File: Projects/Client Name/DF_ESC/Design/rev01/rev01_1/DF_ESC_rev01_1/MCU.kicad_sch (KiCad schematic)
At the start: 11 parts, among them U1 STM32F405RGTx

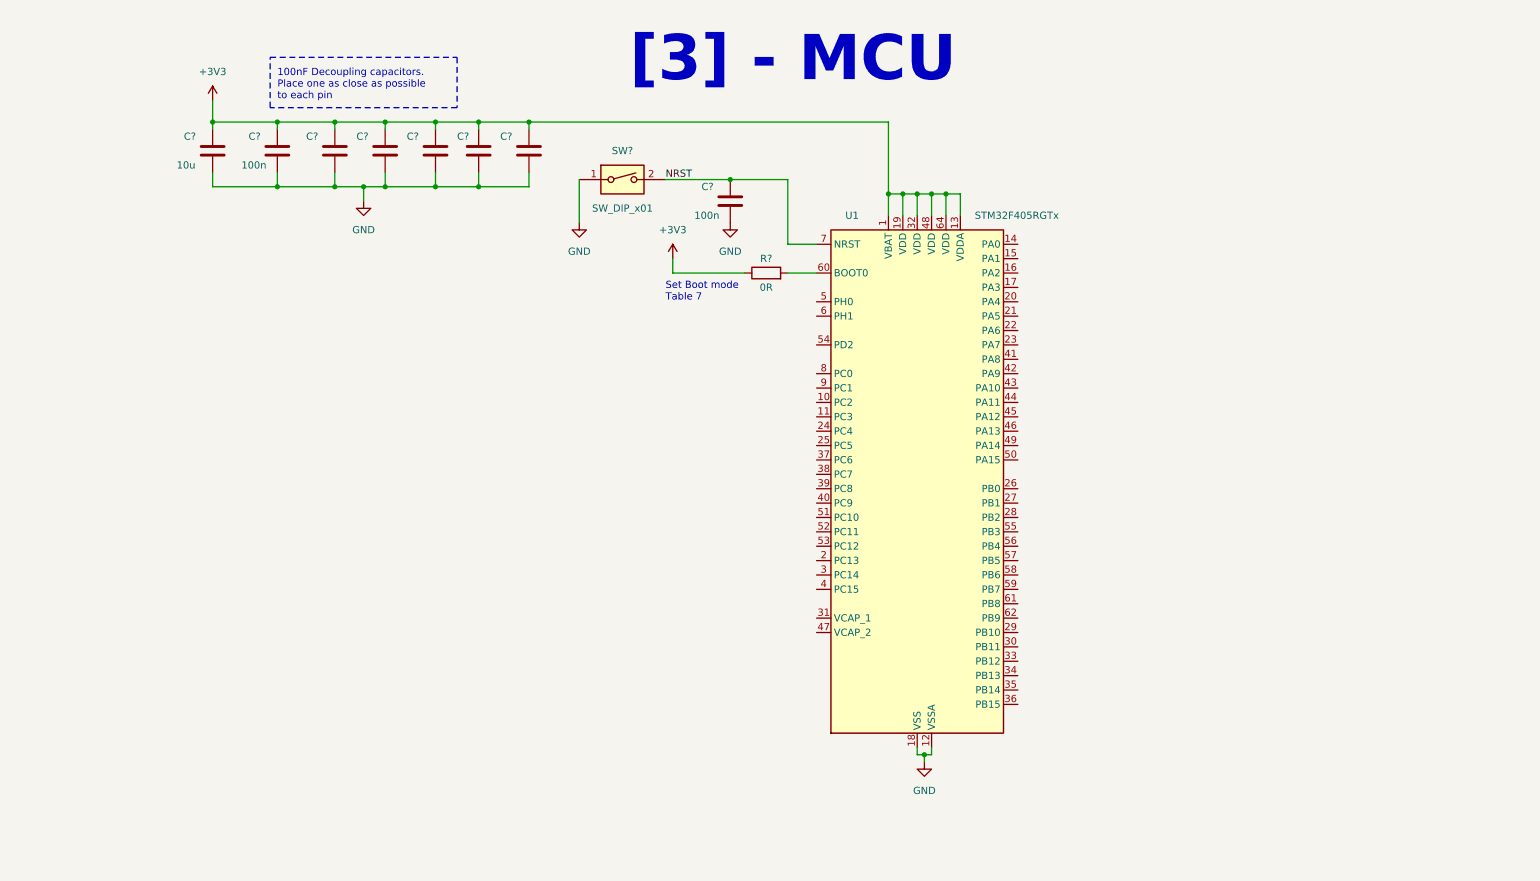
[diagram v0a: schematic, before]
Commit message: Update 19-01-2024_3
MCU schematic complete
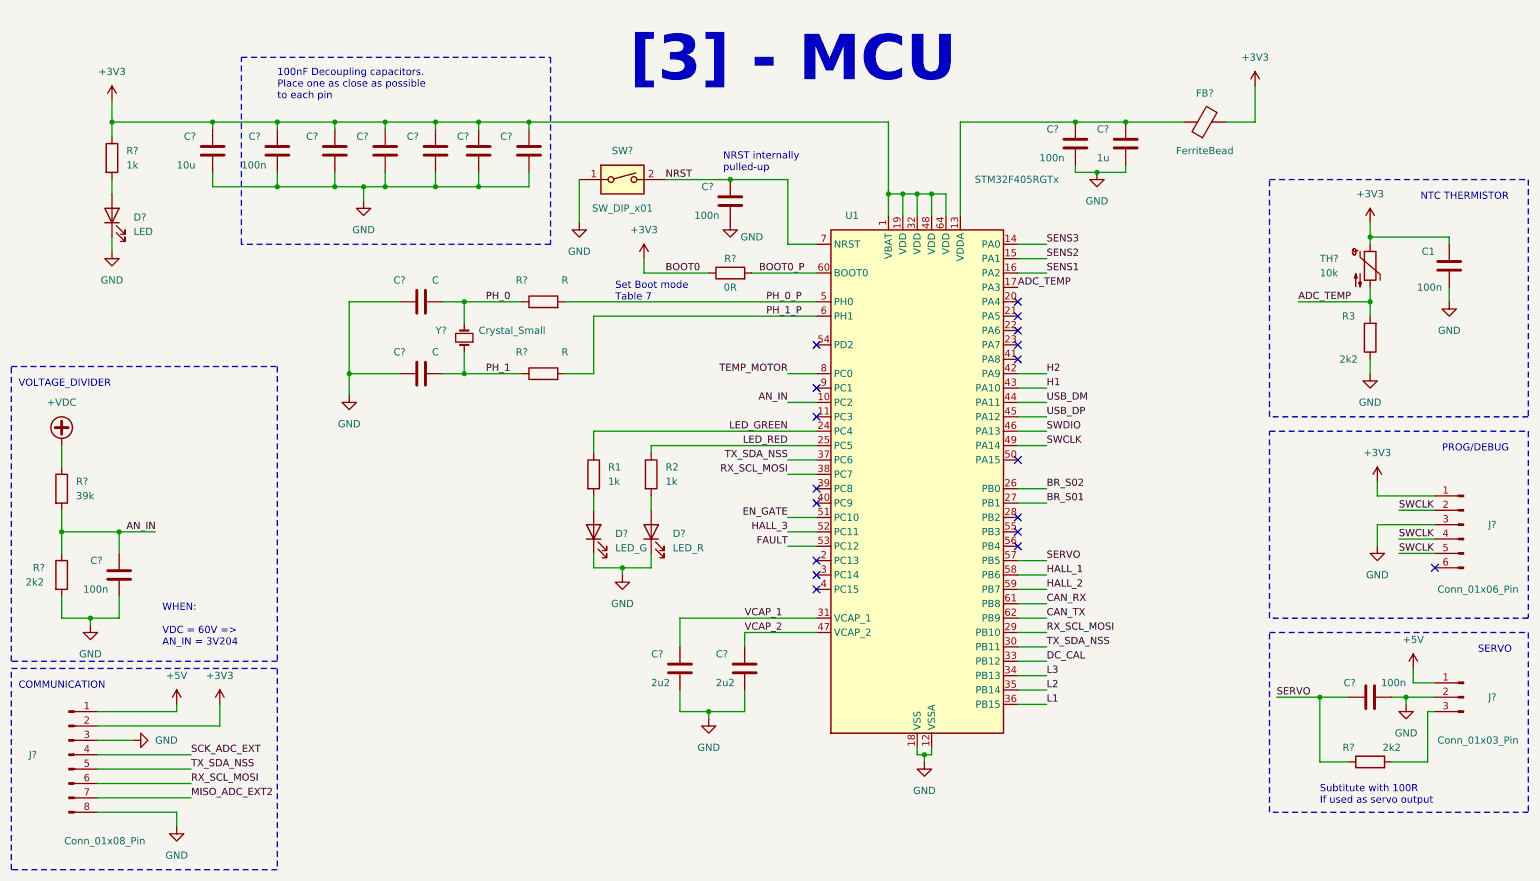
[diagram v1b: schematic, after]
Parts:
- added C1, C? (x3): 100n, symbol Device:C
- added C? (x2): 2u2, symbol Device:C
- added C?: 1u, symbol Device:C
- added C? (x2): C, symbol Device:C
- added D?: LED_G, symbol Device:LED
- added D?: LED_R, symbol Device:LED
- added D?: LED, symbol Device:LED
- added FB?: FerriteBead, symbol Device:FerriteBead
- added J?: Conn_01x03_Pin, symbol Connector:Conn_01x03_Pin
- added J?: Conn_01x08_Pin, symbol Connector:Conn_01x08_Pin
- added J?: Conn_01x06_Pin, symbol Connector:Conn_01x06_Pin
- added R1, R2, R?: 1k, symbol Device:R
- added R3, R? (x2): 2k2, symbol Device:R
- added R?: 39k, symbol Device:R
- added R? (x2): R, symbol Device:R
- added TH?: 10k, symbol Device:Thermistor_NTC
- added Y?: Crystal_Small, symbol Device:Crystal_Small
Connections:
- net +3V3: now also C1.2, FB?.2, J?.1 (Pin_1), J?.2 (Pin_2), R?.1, TH?.1; no longer U1.13 (VDDA)
- net GND: now also C1.1, C?.1, C?.1, C?.2, C?.2, C?.2, C?.2, C?.2, C?.2, D?.1 (K), D?.1 (K), D?.1 (K), J?.2 (Pin_2), J?.3 (Pin_3), J?.3 (Pin_3), J?.8 (Pin_8), R3.1, R?.2
- net BOOT0_P: now reaches R?.2, U1.60 (BOOT0)
- net AN_IN: now reaches U1.10 (PC2)
- net AN_IN: now also C?.1, R?.1, R?.2
- net SENS3: now reaches U1.14 (PA0)
- net SENS2: now reaches U1.15 (PA1)
- net SENS1: now reaches U1.16 (PA2)
- net ADC_TEMP: now reaches U1.17 (PA3)
- net ADC_TEMP: now also R3.2, TH?.2
- net LED_GREEN: now reaches U1.24 (PC4)
- net LED_GREEN: now also R1.1
- net LED_RED: now reaches U1.25 (PC5)
- net LED_RED: now also R2.1
- net BR_S02: now reaches U1.26 (PB0)
- net BR_S01: now reaches U1.27 (PB1)
- net RX_SCL_MOSI: now reaches U1.29 (PB10)
- net RX_SCL_MOSI: now also U1.38 (PC7), J?.6 (Pin_6)
- net TX_SDA_NSS: now reaches U1.30 (PB11)
- net TX_SDA_NSS: now also U1.37 (PC6), J?.5 (Pin_5)
- net VCAP_1: now reaches U1.31 (VCAP_1)
- net VCAP_1: now also C?.1
- net DC_CAL: now reaches U1.33 (PB12)
- net L3: now reaches U1.34 (PB13)
- net L2: now reaches U1.35 (PB14)
- net L1: now reaches U1.36 (PB15)
- net H2: now reaches U1.42 (PA9)
- net H1: now reaches U1.43 (PA10)
- net USB_DM: now reaches U1.44 (PA11)
- net USB_DP: now reaches U1.45 (PA12)
- net SWDIO: now reaches U1.46 (PA13)
- net VCAP_2: now reaches U1.47 (VCAP_2)
- net VCAP_2: now also C?.1
- net SWCLK: now reaches U1.49 (PA14)
- net SWCLK: now also J?.2 (Pin_2), J?.4 (Pin_4), J?.5 (Pin_5)
- net PH_0_P: now reaches U1.5 (PH0)
- net PH_0_P: now also R?.2
- net EN_GATE: now reaches U1.51 (PC10)
- net HALL_3: now reaches U1.52 (PC11)
- net FAULT: now reaches U1.53 (PC12)
- net SERVO: now reaches U1.57 (PB5)
- net SERVO: now also C?.1, R?.1
- net HALL_1: now reaches U1.58 (PB6)
- net HALL_2: now reaches U1.59 (PB7)
- net PH_1_P: now reaches U1.6 (PH1)
- net PH_1_P: now also R?.2
- net CAN_RX: now reaches U1.61 (PB8)
- net CAN_TX: now reaches U1.62 (PB9)
- net TEMP_MOTOR: now reaches U1.8 (PC0)
- new net: J?.3 (Pin_3), R?.2
- new net: C?.1, C?.1, FB?.1, U1.13 (VDDA)
- new net: D?.2 (A), R?.2
- new net: D?.2 (A), R2.2
- new net: D?.2 (A), R1.2
- new net +5V: J?.1 (Pin_1), J?.1 (Pin_1)
- new net +VDC: R?.1
- new net MISO_ADC_EXT2: J?.7 (Pin_7)
- new net PH_0: C?.2, R?.1, Y?.2
- new net PH_1: C?.2, R?.1, Y?.1
- new net SCK_ADC_EXT: J?.4 (Pin_4)
- no-connect marks 0 -> 18
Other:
- note added: "COMMUNICATION"
- note added: "NRST internally pulled-up"
- note added: "NTC THERMISTOR"
- note added: "PROG/DEBUG"
- note added: "SERVO"
- note added: "Subtitute with 100R If used as servo output"
- note added: "VOLTAGE_DIVIDER"
- note added: "WHEN: VDC = 60V => AN_IN = 3V204"
- moved on the sheet: R?
